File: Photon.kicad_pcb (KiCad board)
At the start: 2 copper layers, 21.2 x 74.4 mm, 53 parts, among them J1 USB_C_Receptacle_USB2.0_14P, Q1 IRLML6402, Q2 IRLML6402, SW1 TS-1088-AR02016, U1 ATtiny13A-S, U2 RT8059GJ5, U3 TP4056, U4 BCR421UW6-7, U5 DW01A, U6 FS8205A, U7 BCR421UW6-7

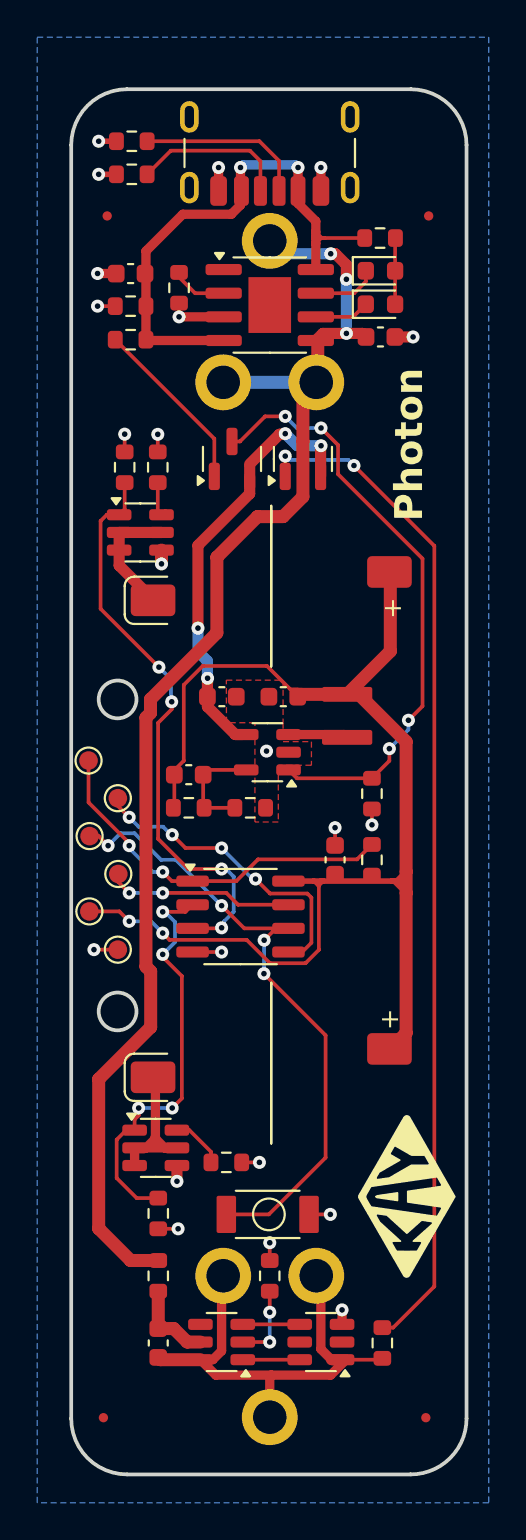
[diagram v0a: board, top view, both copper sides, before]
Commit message: Updated
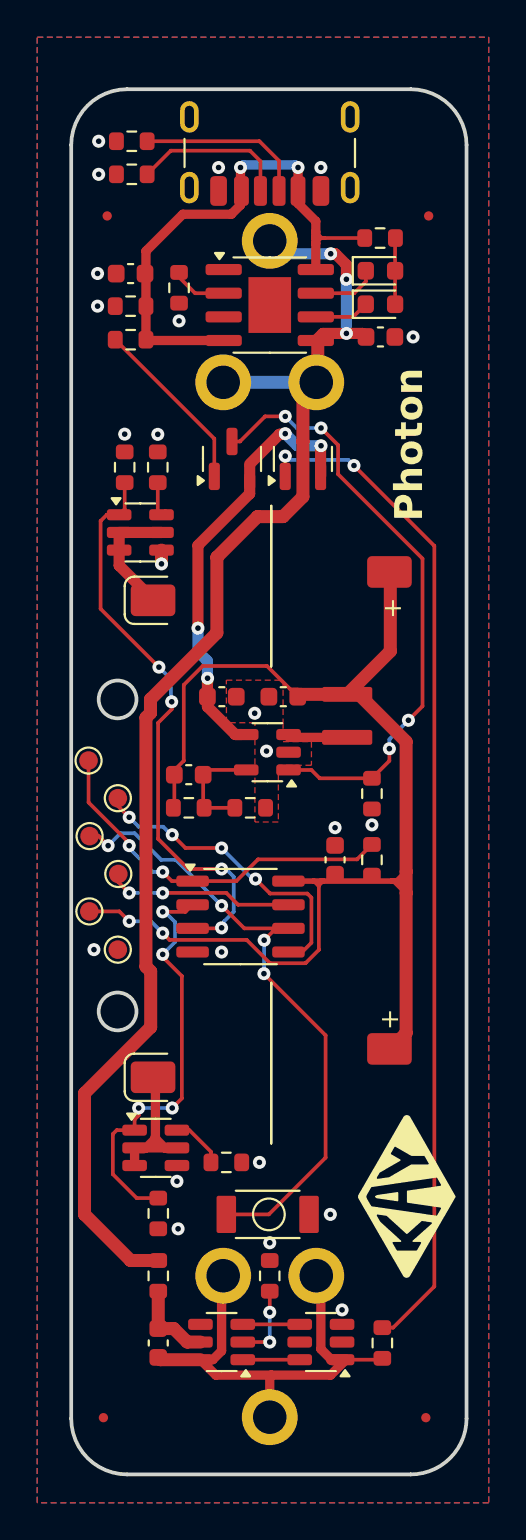
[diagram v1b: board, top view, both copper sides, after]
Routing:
- net GND: track 24.0 -> 0.74 mm, vias 22 -> 23
- net /Bat+: track 73.9 -> 74.5 mm
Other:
- rule pad_to_mask_clearance: 0 -> 0.1
